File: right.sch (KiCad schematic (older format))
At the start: 74 parts, among them J10 UTC16-G, J4 reset, J5 Buzzer, J6 ISP, P6 WS2812, P8 SJ-43514-SMT, SW25 Socket, SW26 Socket, SW27 Socket, SW28 Socket, SW29 Socket, SW30 Socket, SW31 Socket, SW32 Socket, SW33 Socket, SW34 Socket, SW35 Socket, SW36 Socket, SW37 Socket, SW38 Socket, SW39 Socket, SW40 Socket, SW41 Socket, SW42 Socket, SW43 Socket, SW44 Socket, SW45 Socket, SW46 Socket, SW47 Socket, SW48 Socket, SW50 FSMSM, U2 ATMega32U4, Y2 16MHz

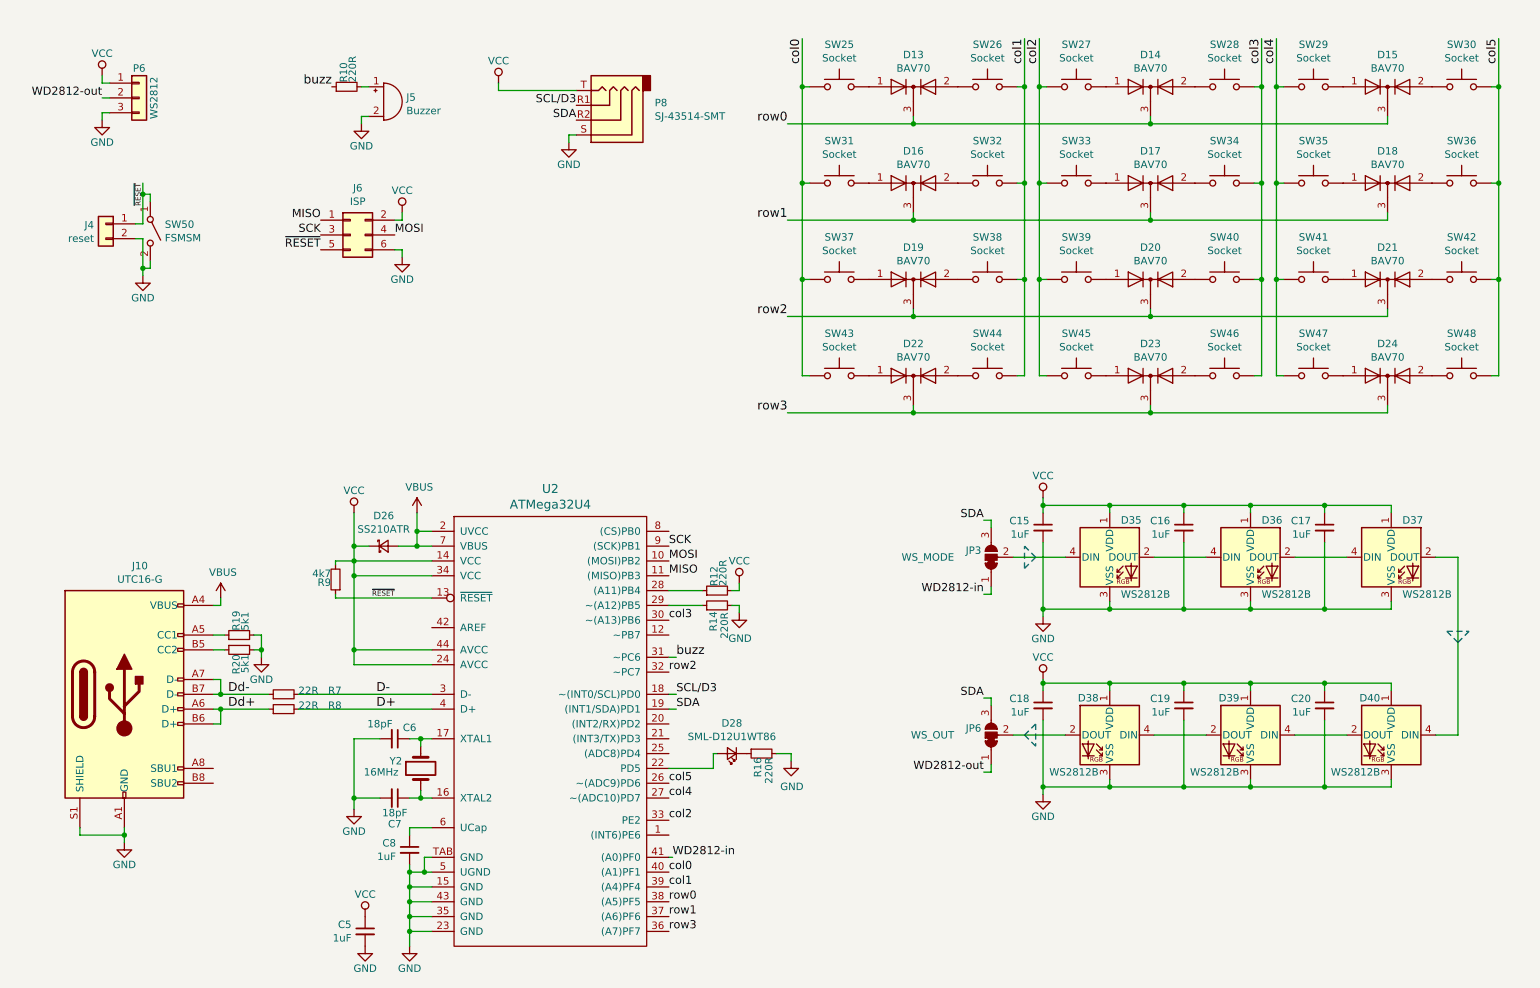
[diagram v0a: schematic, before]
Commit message: Pre-cleanup
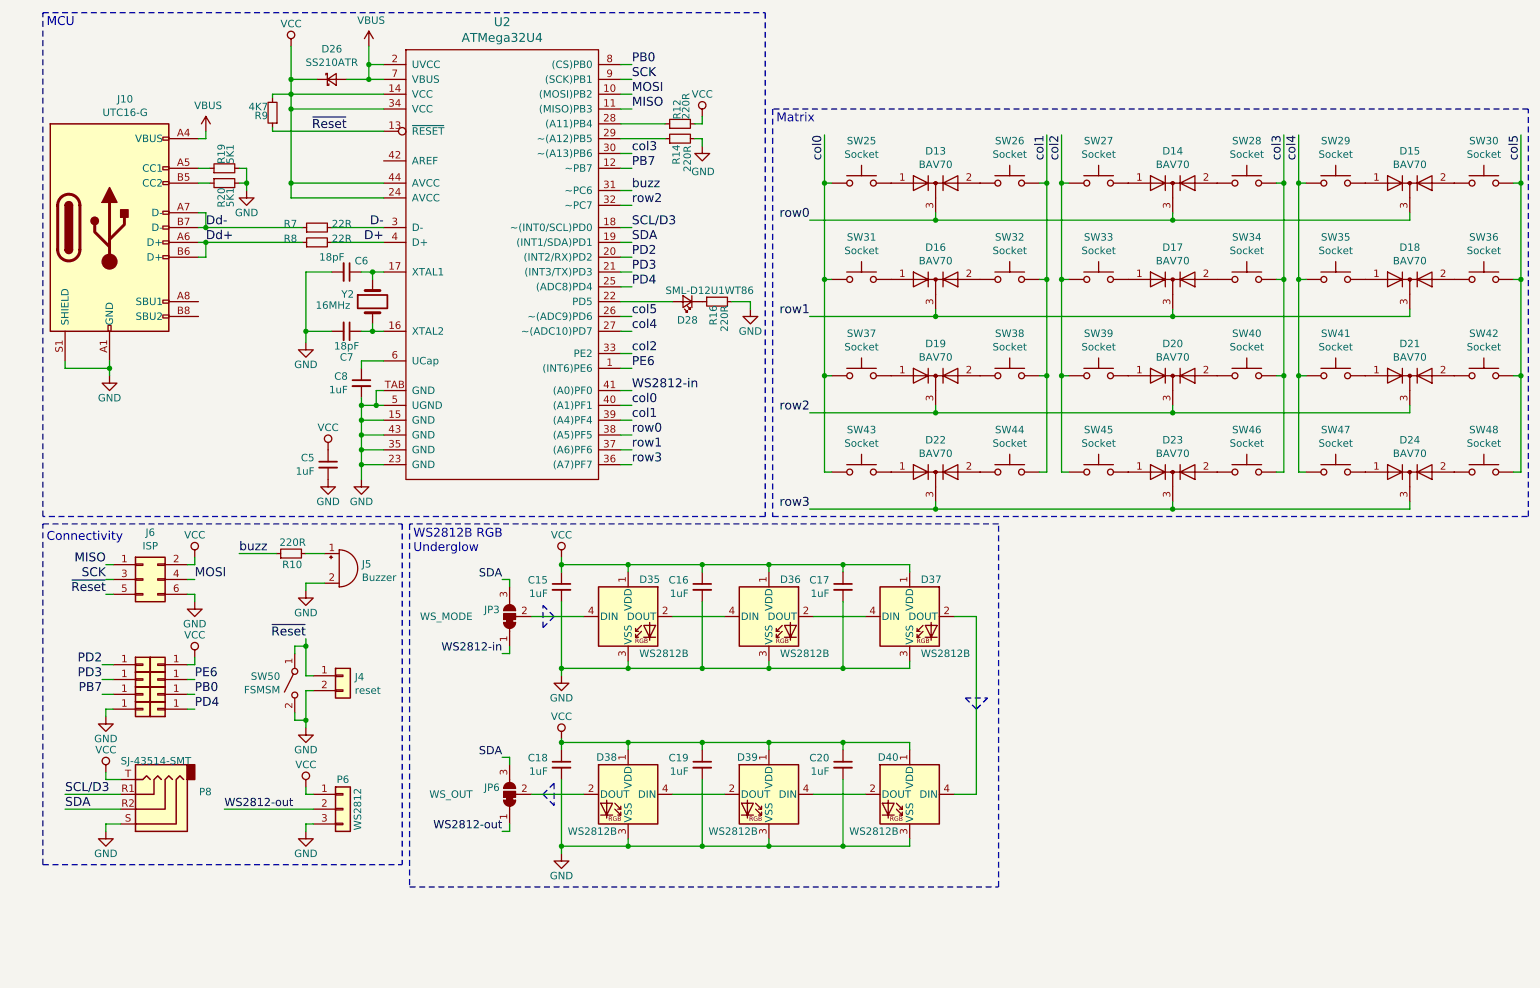
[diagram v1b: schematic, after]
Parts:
- added J18, J19, J20, J21, J22, J23, J24, J8: Conn_01x01, TestPoint:TestPoint_Pad_D1.5mm, symbol Connector_Generic:Conn_01x01
- R19, R20: value 5k1 -> 5K1
- R9: value 4k7 -> 4K7
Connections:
- net GND: now also J23.1 (Pin_1)
- net VCC: now also J18.1 (Pin_1)
- net PE6: now reaches U2.1 ((INT6)PE6)
- net PE6: now also J20.1 (Pin_1)
- net PB7: now reaches U2.12 (~~PB7)
- net PB7: now also J21.1 (Pin_1)
- net PD2: now reaches U2.20 ((INT2/RX)PD2)
- net PD2: now also J8.1 (Pin_1)
- net PD3: now reaches U2.21 ((INT3/TX)PD3)
- net PD3: now also J19.1 (Pin_1)
- net PD4: now reaches U2.25 ((ADC8)PD4)
- net PD4: now also J24.1 (Pin_1)
- net PB0: now reaches U2.8 ((CS)PB0)
- net PB0: now also J22.1 (Pin_1)
- net WD2812-in renamed WS2812-in
- net WD2812-out renamed WS2812-out
- net ~RESET renamed ~Reset
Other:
- note added: "Connectivity"
- note added: "MCU"
- note added: "Matrix"
- note added: "WS2812B RGB\nUnderglow"
- moved on the sheet: C15, C16, C17, C18, C19, C20, C5, C6, C7, C8, D13, D14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
